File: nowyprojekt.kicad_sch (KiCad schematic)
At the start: 42 parts, among them J1 Zasilanie, J2 01x03, J3 Conn_01x15_Pin, J4 Conn_01x15_Pin, Q1 BC856, Q2 BC856, Q3 BC856, Q4 BC856, U1 CA56-12SURKWA, U2 ATMEGA328P-AU, U3 AMS1117-5.0

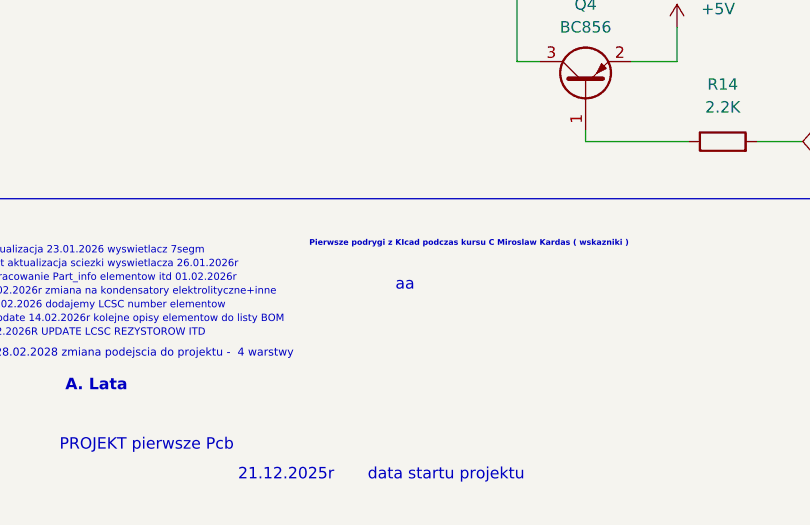
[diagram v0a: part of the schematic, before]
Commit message: --
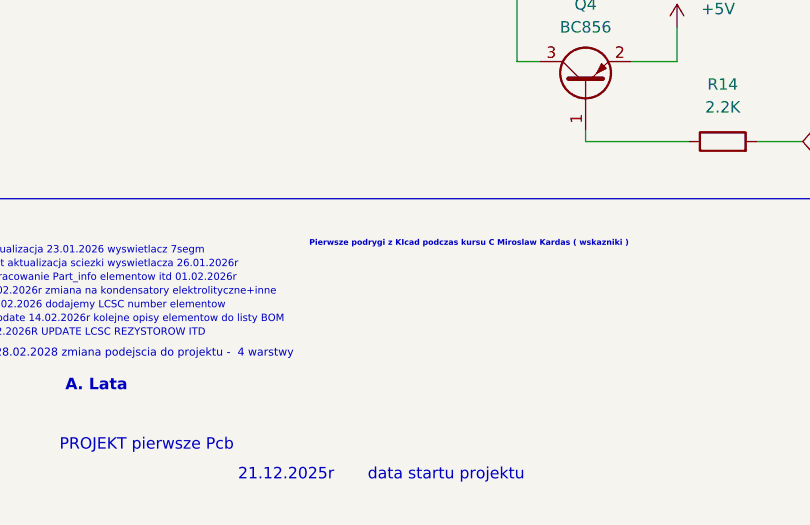
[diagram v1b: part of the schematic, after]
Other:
- note removed: "aa"
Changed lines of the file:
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@@
-		)
-	)
-	(text "aa"
-		(exclude_from_sim no)
-		(at 226.314 172.212 0)
-		(effects
-			(font
-				(size 1.27 1.27)
-			)
 		)
 	)

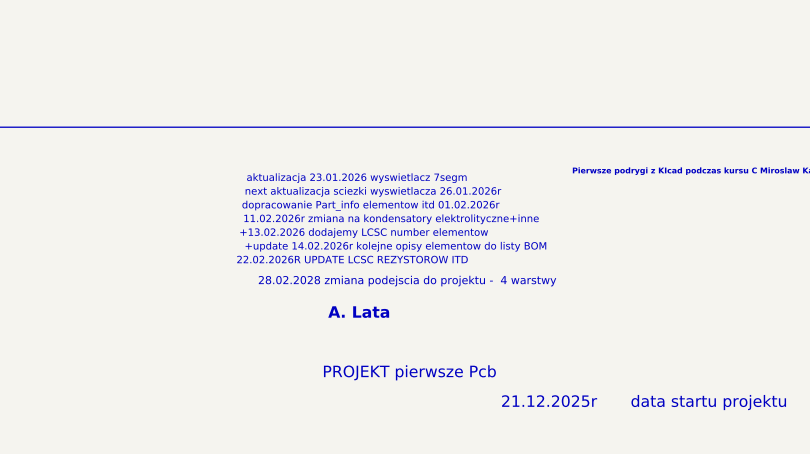
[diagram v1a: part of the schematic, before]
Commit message: maly update02.03.2026r
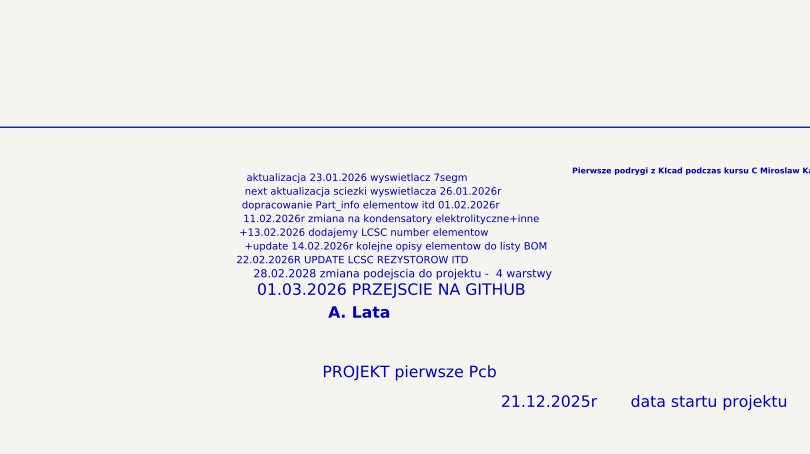
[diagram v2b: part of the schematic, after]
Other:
- note added: "01.03.2026 PRZEJSCIE NA GITHUB"
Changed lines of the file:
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@@
+		)
+	)
+	(text "01.03.2026 PRZEJSCIE NA GITHUB"
+		(exclude_from_sim no)
+		(at 195.58 180.848 0)
+		(effects
+			(font
+				(size 1.27 1.27)
+			)
 		)
 	)
@@
 	(text "28.02.2028 zmiana podejscia do projektu -  4 warstwy "
 		(exclude_from_sim no)
-		(at 197.358 179.832 0)
+		(at 196.85 179.07 0)
 		(effects
 			(font
